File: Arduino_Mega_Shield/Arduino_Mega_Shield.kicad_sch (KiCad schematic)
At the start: 46 parts, among them J1 Conn_01x04, J10 SW10, J11 SW6, J12 SW7, J13 SW8, J14 SW9, J15 Motor Driver Connector, J16 Motor Driver Connector, J17 Motor Driver Connector, J18 Motor Driver Connector, J19 Screw_Terminal_01x02, J2 Conn_01x04, J20 JOYSTICK, J21 I2C CONNECTOR, J22 ENCODER1, J23 ENCODER2, J24 ENCODER3, J25 ENCODER4, J26 UART CONNECTOR, J3 Conn_01x04, J4 Conn_01x04, J5 SW5, J6 SW1, J7 SW2, J8 SW3, J9 SW4

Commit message: Avancement on the electric shemas and some fixe on the PCB
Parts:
- added J27, J28, J29, J30, J31, J32, J33, J34, J35, J36, J37, J38: 3_pin_selector, Arduino MCU:3 pin selector, symbol Motor_controller:3_pin_selector
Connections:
- net +12V: now also A1.8 (VMOT), A2.8 (VMOT), A3.8 (VMOT), A4.8 (VMOT)
- net +5V: now also A1.2 (VDD), A2.2 (VDD), A3.2 (VDD), A4.2 (VDD), J27.1 (Pin_1), J28.1 (Pin_1), J29.1 (Pin_1), J30.1 (Pin_1), J31.1 (Pin_1), J32.1 (Pin_1), J33.1 (Pin_1), J34.1 (Pin_1), J35.1 (Pin_1), J36.1 (Pin_1), J37.1 (Pin_1), J38.1 (Pin_1)
- net ENC_A1: now also A5.D2 (D2_INT0)
- net ENC_A2: now also A5.D3 (D3_INT1)
- net GND: now also A1.1 (GND), A1.7 (GND), A2.1 (GND), A2.7 (GND), A3.1 (GND), A3.7 (GND), A4.1 (GND), A4.7 (GND), J27.3 (Pin_3), J28.3 (Pin_3), J29.3 (Pin_3), J30.3 (Pin_3), J31.3 (Pin_3), J32.3 (Pin_3), J33.3 (Pin_3), J34.3 (Pin_3), J35.3 (Pin_3), J36.3 (Pin_3), J37.3 (Pin_3), J38.3 (Pin_3)
- net LPWM1: now also A1.16 (DIR)
- net LPWM2: now also A2.16 (DIR)
- net LPWM3: now also A3.16 (DIR)
- net LPWM4: now also A4.16 (DIR)
- net L_IS1: now also A1.14 (~{SLEEP})
- net L_IS2: now also A2.14 (~{SLEEP})
- net L_IS3: now also A3.14 (~{SLEEP})
- net L_IS4: now also A4.14 (~{SLEEP})
- net RPWM1: now also A1.15 (STEP)
- net RPWM2: now also A2.15 (STEP)
- net RPWM3: now also A3.15 (STEP)
- net RPWM4: now also A4.15 (STEP)
- net R_EN1: now also A1.9 (~{ENABLE})
- net R_EN2: now also A2.9 (~{ENABLE})
- net R_EN3: now also A3.9 (~{ENABLE})
- net R_EN4: now also A4.9 (~{ENABLE})
- net R_IS1: now also A1.13 (~{RESET})
- net R_IS2: now also A2.13 (~{RESET})
- net R_IS3: now also A3.13 (~{RESET})
- net R_IS4: now also A4.13 (~{RESET})
- net at A4.10 (MS1): now also J38.2 (Pin_2)
- net at A4.11 (MS2): now also J37.2 (Pin_2)
- net at A4.12 (MS3): now also J36.2 (Pin_2)
- net at A3.10 (MS1): now also J35.2 (Pin_2)
- net at A3.11 (MS2): now also J34.2 (Pin_2)
- net at A3.12 (MS3): now also J33.2 (Pin_2)
- net at A1.10 (MS1): now also J29.2 (Pin_2)
- net at A1.11 (MS2): now also J28.2 (Pin_2)
- net at A1.12 (MS3): now also J27.2 (Pin_2)
- net at A2.10 (MS1): now also J32.2 (Pin_2)
- net at A2.11 (MS2): now also J31.2 (Pin_2)
- net at A2.12 (MS3): now also J30.2 (Pin_2)
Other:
- moved on the sheet: A2, A3, A4, A5, BZ1, D1, J10, J11, J12, J13, J14, J15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

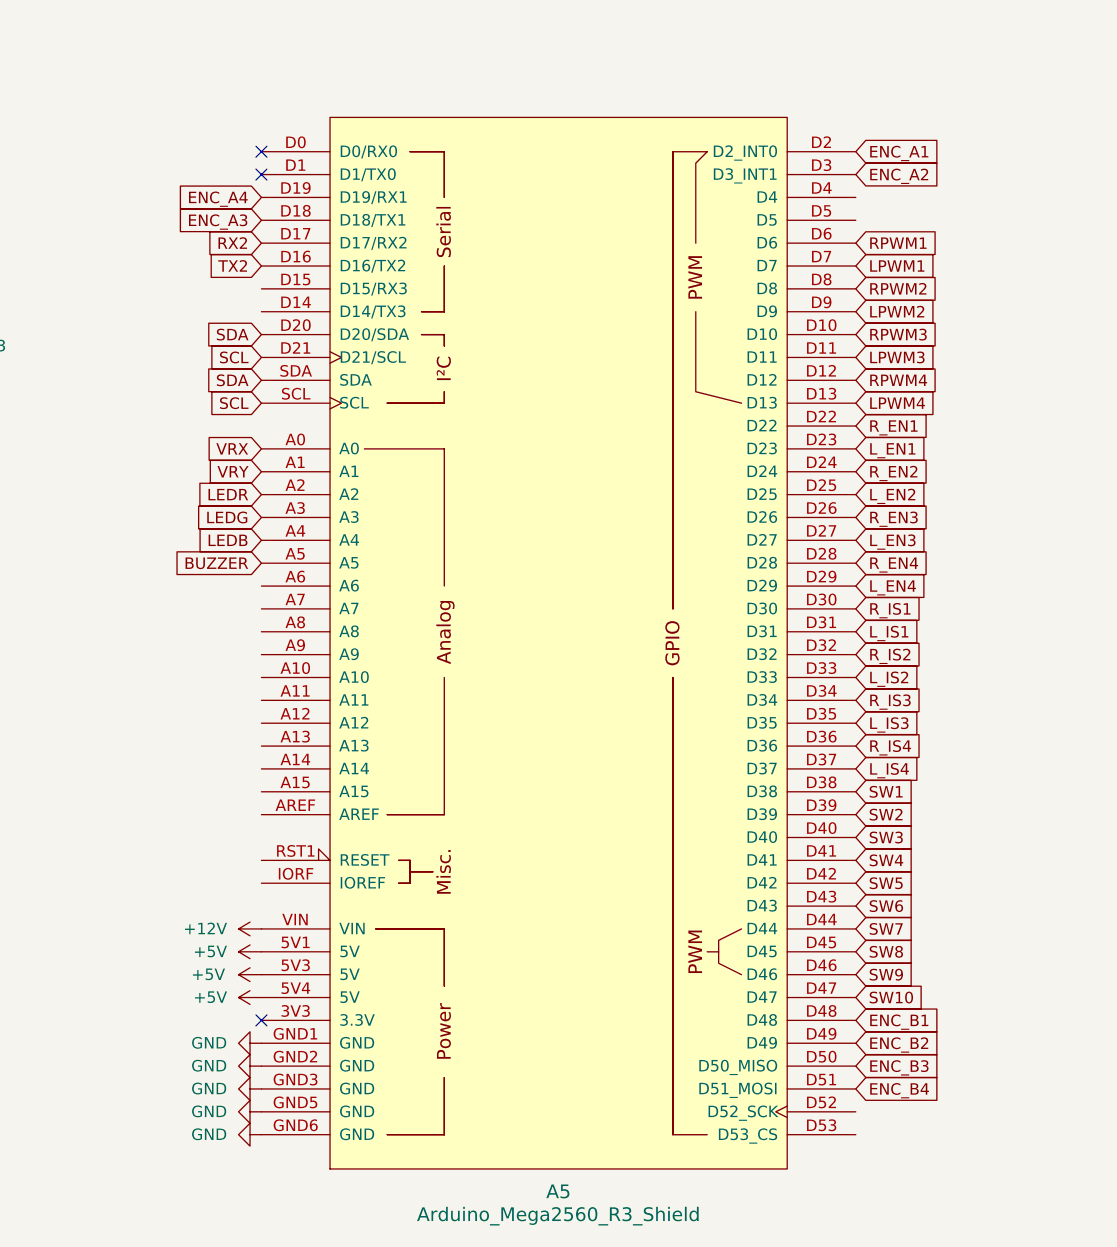
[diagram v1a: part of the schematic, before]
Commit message: Avancement in the PCB design
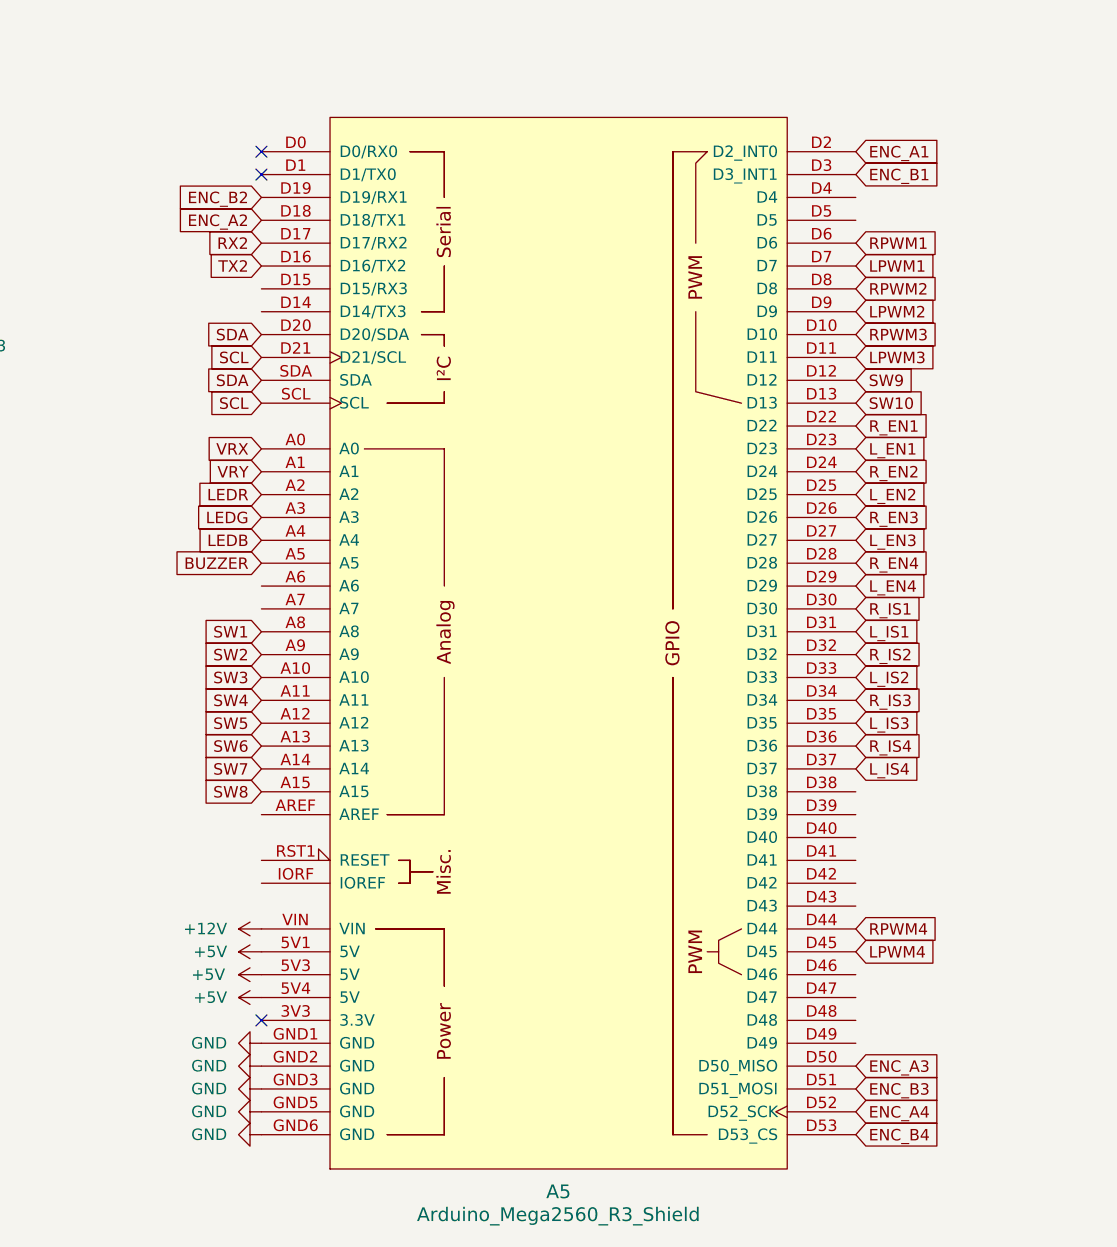
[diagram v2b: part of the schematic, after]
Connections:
- net ENC_A2: now also A5.D18 (D18/TX1); no longer A5.D3 (D3_INT1)
- net ENC_A3: now also A5.D50 (D50_MISO); no longer A5.D18 (D18/TX1)
- net ENC_A4: now also A5.D52 (D52_SCK); no longer A5.D19 (D19/RX1)
- net ENC_B1: now also A5.D3 (D3_INT1); no longer A5.D48
- net ENC_B2: now also A5.D19 (D19/RX1); no longer A5.D49
- net ENC_B3: now also A5.D51 (D51_MOSI); no longer A5.D50 (D50_MISO)
- net ENC_B4: now also A5.D53 (D53_CS); no longer A5.D51 (D51_MOSI)
- net LPWM4: now also A5.D45; no longer A5.D13
- net RPWM4: now also A5.D44; no longer A5.D12
- net SW1: now also A5.A8; no longer A5.D38
- net SW10: now also A5.D13; no longer A5.D47
- net SW2: now also A5.A9; no longer A5.D39
- net SW3: now also A5.A10; no longer A5.D40
- net SW4: now also A5.A11; no longer A5.D41
- net SW5: now also A5.A12; no longer A5.D42
- net SW6: now also A5.A13; no longer A5.D43
- net SW7: now also A5.A14; no longer A5.D44
- net SW8: now also A5.A15; no longer A5.D45
- net SW9: now also A5.D12; no longer A5.D46
